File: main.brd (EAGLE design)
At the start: 100 x 80 mm, 23 parts, among them U1 ATMEGA328P_TQFP

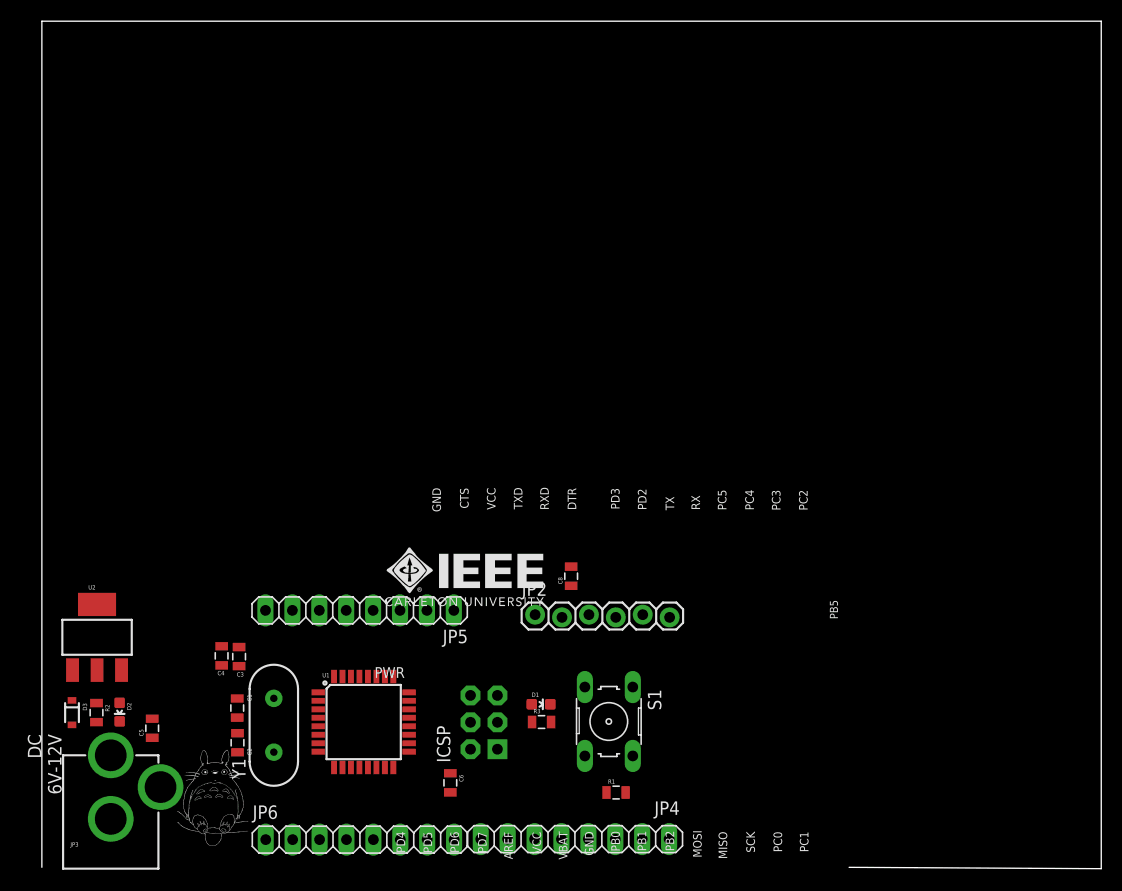
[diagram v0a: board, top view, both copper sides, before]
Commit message: Board layout made
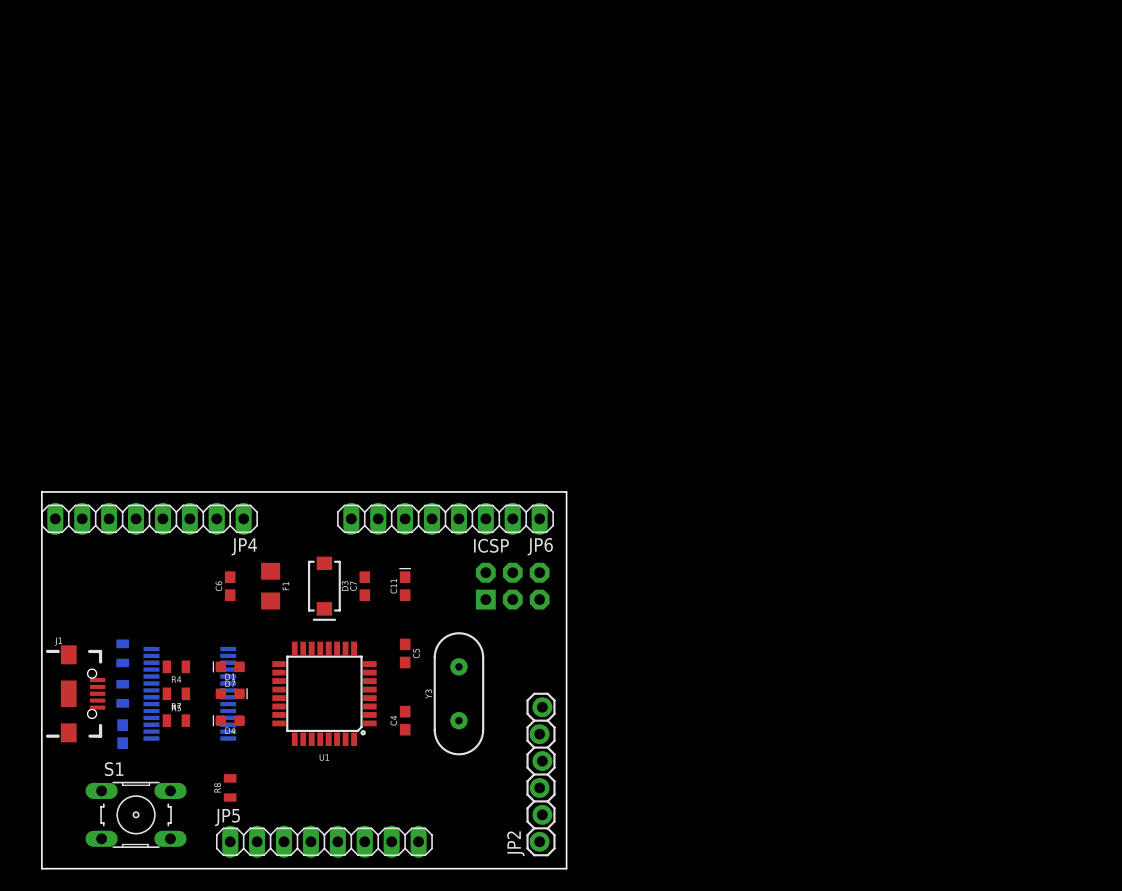
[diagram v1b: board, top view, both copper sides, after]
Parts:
- removed C1, C3, C8: (no value), SparkFun-Passives:0805
- removed D2: BLUE, SparkFun-LED:LED-0603
- removed JP3: POWER_JACKPTH, SparkFun-Connectors:POWER_JACK_PTH
- removed R1: (no value), SparkFun-Resistors:0805
- removed U2: (no value), SparkFun-PowerIC:SOT223
- removed Y1: (no value), SparkFun-FreqCtrl:HC49US
- added C11: 4.7uF, SparkFun-Capacitors:0603-POLAR
- added C7: 0.1uF, SparkFun-Capacitors:0603
- added D4: RED, SparkFun-LED:LED-0603
- added D7: GREEN, SparkFun-LED:LED-0603
- added F1: 6V/0.5A, SparkFun-Fuses:1206
- added IC1: FT232RL, ftdichip:SSOP28
- added J1: (no value), SparkFun-Connectors:USB-B-MICRO-SMD
- added R4, R5, R7, R8: 1k, SparkFun-Resistors:0805
- added Y3: 16MHz, SparkFun-Clocks:HC49US
- C2, C6: value (none) -> 0.1uF; device SparkFun-Passives:0805 -> SparkFun-Capacitors:0603
- C4, C5: value (none) -> 22pF; device SparkFun-Passives:0805 -> SparkFun-Capacitors:0603
- D3: value 250mA/100V -> 2A/100V/850mV; device SparkFun-DiscreteSemi:SOD-323 -> SparkFun-DiscreteSemi:SMA-DIODE
- R2, R3: value (none) -> 1k
- U1: device SparkFun-DigitalIC:TQFP32-08 -> SparkFun-IC-Microcontroller:TQFP32-08
- moved JP4 50.3 mm to (10.2, 33.0), turned to 180 degrees
- moved S1 45.5 mm to (8.89, 5.08), turned to 0 degrees
- moved R3 40.1 mm to (7.62, 20.3), flipped to the bottom, turned to 90 degrees
- moved JP6 31.3 mm to (38.1, 33.0), turned to 180 degrees
- moved D1 29.5 mm to (17.8, 19.1), turned to 180 degrees
- moved C6 27.9 mm to (17.8, 26.7), turned to 90 degrees
- moved D3 26.6 mm to (26.7, 26.7)
- moved C5 24.9 mm to (34.3, 20.3), turned to 270 degrees
- moved JP5 22.1 mm to (26.7, 2.54), turned to 0 degrees
- moved JP2 21.4 mm to (47.0, 2.54), turned to 90 degrees
- moved C4 18.4 mm to (34.3, 14.0)
- moved ICSP 13.1 mm to (44.5, 26.7), turned to 0 degrees
- moved C2 10.9 mm to (7.62, 12.7), flipped to the bottom
- moved U1 4.57 mm to (26.7, 16.5), turned to 180 degrees
- moved R2 3.04 mm to (7.62, 16.5), flipped to the bottom
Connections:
- removed net N$4: D1.A, R3.1
- removed net N$5: C8.2, JP2.1
- new net 3.3V: C6.2, IC1.17
- new net 5V: D1.A, D3.C, D4.A, R2.2, R3.2, R7.2, R8.2
- new net CBUS0: IC1.23, R2.1
- new net CBUS1: IC1.22, R3.1
- new net N$15: IC1.20, IC1.4
- new net N$17: U1.21, U1.3, U1.5
- new net N$19: J1.GND
- new net N$20: J1.SHIELD1, J1.SHIELD2, J1.SHIELD3
- new net N$21: IC1.18, IC1.21, IC1.26, IC1.7
- new net N$22: IC1.25
- new net N$7: C2.2, IC1.19
- new net USBD+: IC1.15, J1.D+
- new net USBD-: IC1.16, J1.D-
- new net VBUS: F1.2, J1.VBUS
- new net V_USB: C11.+, C7.2, D3.A, F1.1
- net GND: now also C11.-, C4.1, C5.1, C6.1, C7.1, D7.C; no longer C1.2, C2.2, C3.2, C4.2, C5.2, C6.2, D1.C, D2.C, D3.A, JP3.GND, JP3.GNDBREAK, U1.21, U1.3, U1.5, U2.1
- net N$3: now also D7.A, R7.1; no longer D2.A, R2.1
- net RST: now also C2.1, JP2.1, R8.1; no longer C8.1, R1.1
- net RX: now also D1.C, IC1.1, R4.1, R4.2
- net SCK: no longer R3.2
- net TX: now also D4.C, IC1.5, R5.1, R5.2
- net VBAT: no longer C5.1, JP3.PWR, U2.3
- net VCC: no longer C3.1, C4.1, C6.1, D3.C, R1.2, R2.2, U2.2, U2.4
- net XTAL_N: now also C5.2, Y3.2; no longer C2.1, Y1.1
- net XTAL_P: now also C4.2, Y3.1; no longer C1.1, Y1.2
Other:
- board size 100 x 80 mm -> 49.5 x 35.6 mm
- board text removed: "AREF"
- board text removed: "CTS"
- board text removed: "DC 6V-12V"
- board text removed: "DTR"
- board text removed: "GND"
- board text removed: "Hasith Vidanamadura hasith@vidanamadura.net, 2015"
- board text removed: "MISO"
- board text removed: "MOSI"
- board text removed: "PB0"
- board text removed: "PB1"
- board text removed: "PB2"
- board text removed: "PB5"
- board text removed: "PC0"
- board text removed: "PC1"
- board text removed: "PC2"
- board text removed: "PC3"
- board text removed: "PC4"
- board text removed: "PC5"
- board text removed: "PD2"
- board text removed: "PD3"
- board text removed: "PD4"
- board text removed: "PD5"
- board text removed: "PD6"
- board text removed: "PD7"
- board text removed: "PWR"
- board text removed: "RX"
- board text removed: "RXD"
- board text removed: "SCK"
- board text removed: "TX"
- board text removed: "TXD"
- board text removed: "VBAT"
- board text removed: "VCC"
